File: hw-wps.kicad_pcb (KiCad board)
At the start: 2 copper layers, 65 x 56 mm, 16 parts, among them J1 GPIO, J2 Screw_Terminal_01x03, U1 ESP32DevKitv1

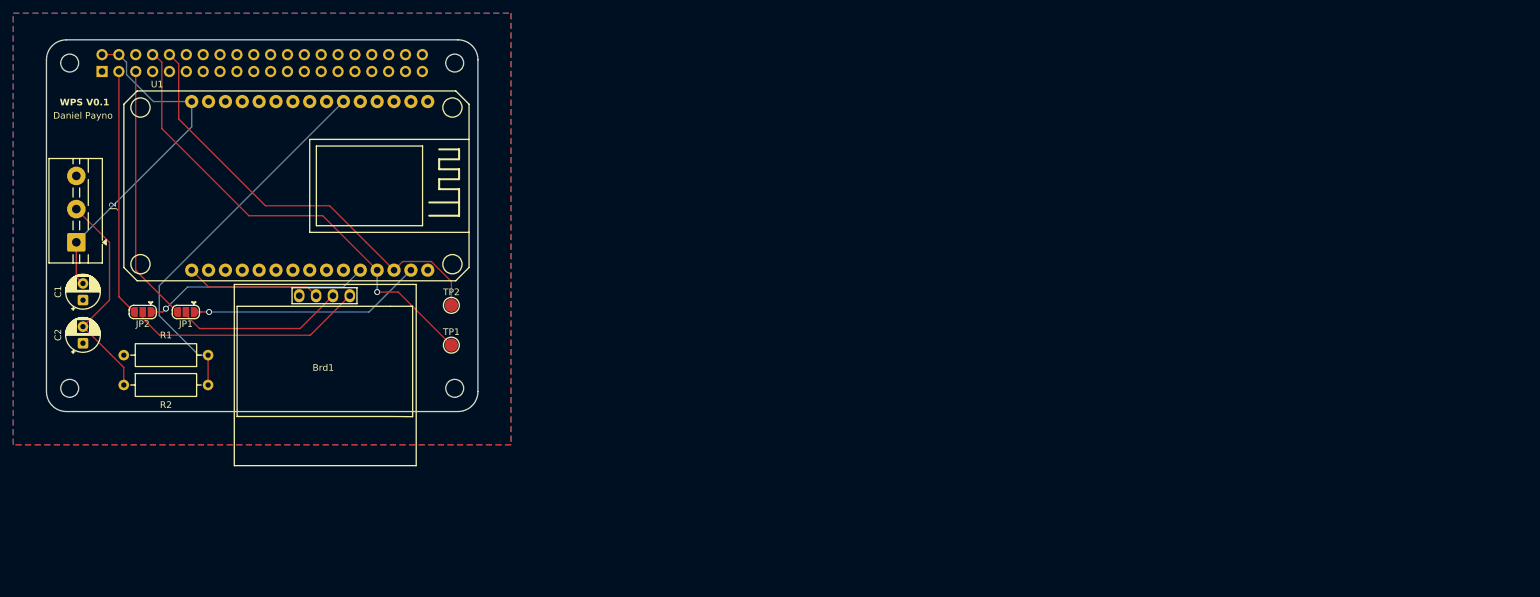
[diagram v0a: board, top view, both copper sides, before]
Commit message: Release v0.2
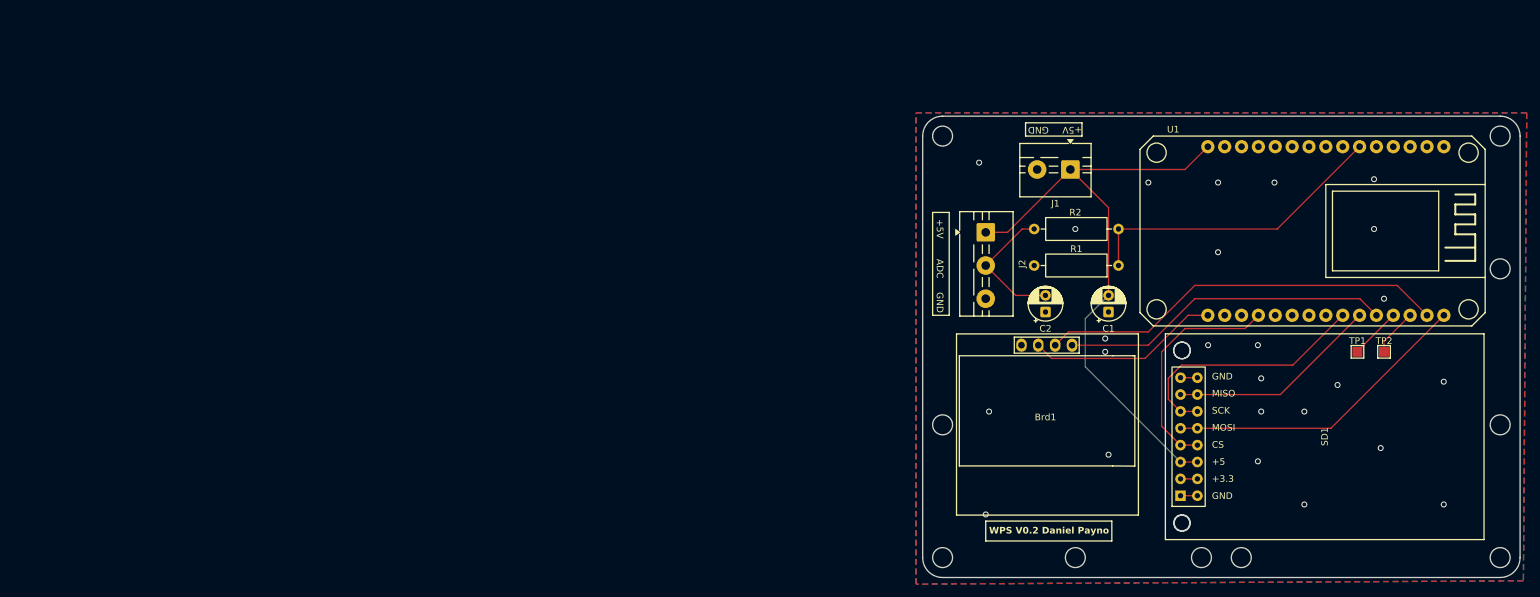
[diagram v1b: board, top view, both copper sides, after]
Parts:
- removed JP1, JP2: SolderJumper_3_Open, Jumper:SolderJumper-3_P1.3mm_Open_RoundedPad1.0x1.5mm
- removed MH1, MH2, MH3, MH4: MountingHole_2.7mm_M2.5, MountingHole:MountingHole_2.7mm_M2.5
- added SD1: SD card reader, SD_card_I2C:SD_card_I2C, F.Cu at (316.6, 119.3)
- J1: value GPIO -> Screw_Terminal_01x02; footprint Connector_PinSocket_2.54mm:PinSocket_2x20_P2.54mm_Vertical -> TerminalBlock:TerminalBlock_MaiXu_MX126-5.0-02P_1x02_P5.00mm; moved to F.Cu
- TP1, TP2: footprint TestPoint:TestPoint_Pad_D2.0mm -> TestPoint:TestPoint_Pad_1.5x1.5mm
- moved C1 154.5 mm to (260.0, 85.0)
- moved U1 153.2 mm to (292.7, 72.8)
- moved J1 146.6 mm to (254.2, 63.5), turned to 180 degrees
- moved C2 145.1 mm to (250.5, 85.0)
- moved TP2 140.7 mm to (301.5, 91.0)
- moved R2 139.1 mm to (248.8, 72.5)
- moved R1 137.8 mm to (261.5, 78.0)
- moved J2 137.0 mm to (241.5, 73.0), turned to -90 degrees
- moved TP1 136.5 mm to (297.5, 91.0)
- moved Brd1 109.1 mm to (250.5, 100.6)
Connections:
- J1 pad 1: +3V3 -> +5V
- J1 pad 2: +5V -> GND
- TP1 pad 1: /GPIO14/TXD0 -> Net-(U1-RX0/D3)
- TP2 pad 1: /GPIO15/RXD0 -> Net-(U1-TX0/D1)
- U1 pad 10: unconnected-(U1-D19-Pad10) -> /MISO
- U1 pad 11: /SDA_ESP32 -> /SDA
- U1 pad 12: /GPIO14/TXD0 -> Net-(U1-RX0/D3)
- U1 pad 13: /GPIO15/RXD0 -> Net-(U1-TX0/D1)
- U1 pad 14: /SCL_ESP32 -> /SCL
- U1 pad 15: unconnected-(U1-D23-Pad15) -> /MOSI
- U1 pad 4: unconnected-(U1-D2-Pad4) -> /CS
- U1 pad 9: unconnected-(U1-D18-Pad9) -> /SCK
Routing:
- net /GPIO14/TXD0: track 71.3 -> 0.00 mm, vias 1 -> 0
- net /GPIO15/RXD0: track 66.2 -> 0.00 mm
- net /MOSI: track 0.00 -> 46.7 mm
- net +5V: track 52.5 -> 95.2 mm
- net /GPIO3/SCL1: track 38.8 -> 0.00 mm
- net /SCK: track 0.00 -> 38.5 mm
- net /GPIO2/SDA1: track 38.0 -> 0.00 mm
- net /SCL: track 25.5 -> 61.6 mm
- net /SCL_ESP32: track 35.3 -> 0.00 mm, vias 1 -> 0
- net /CS: track 0.00 -> 34.6 mm
- net /SDA_ESP32: track 34.1 -> 0.00 mm, vias 1 -> 0
- net /MISO: track 0.00 -> 31.9 mm
- net /SDA: track 36.1 -> 49.8 mm
- net /ADC_IN: track 32.8 -> 20.4 mm
- net Net-(U1-D32): track 58.1 -> 47.0 mm
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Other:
- board size 65 x 56 mm -> 90 x 69.5 mm
- board text added: "+5V"
- board text added: "ADC"
- board text added: "GND"
- board text added: "WPS V0.2 Daniel Payno"
- board text removed: "Daniel Payno"
- board text removed: "Extend PCB edge 0.5mm if using SMT header"
- board text removed: "PoE"
- board text removed: "RJ45"
- board text removed: "USB"
- board text removed: "WPS V0.1"
